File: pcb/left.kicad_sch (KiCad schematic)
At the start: 0 parts

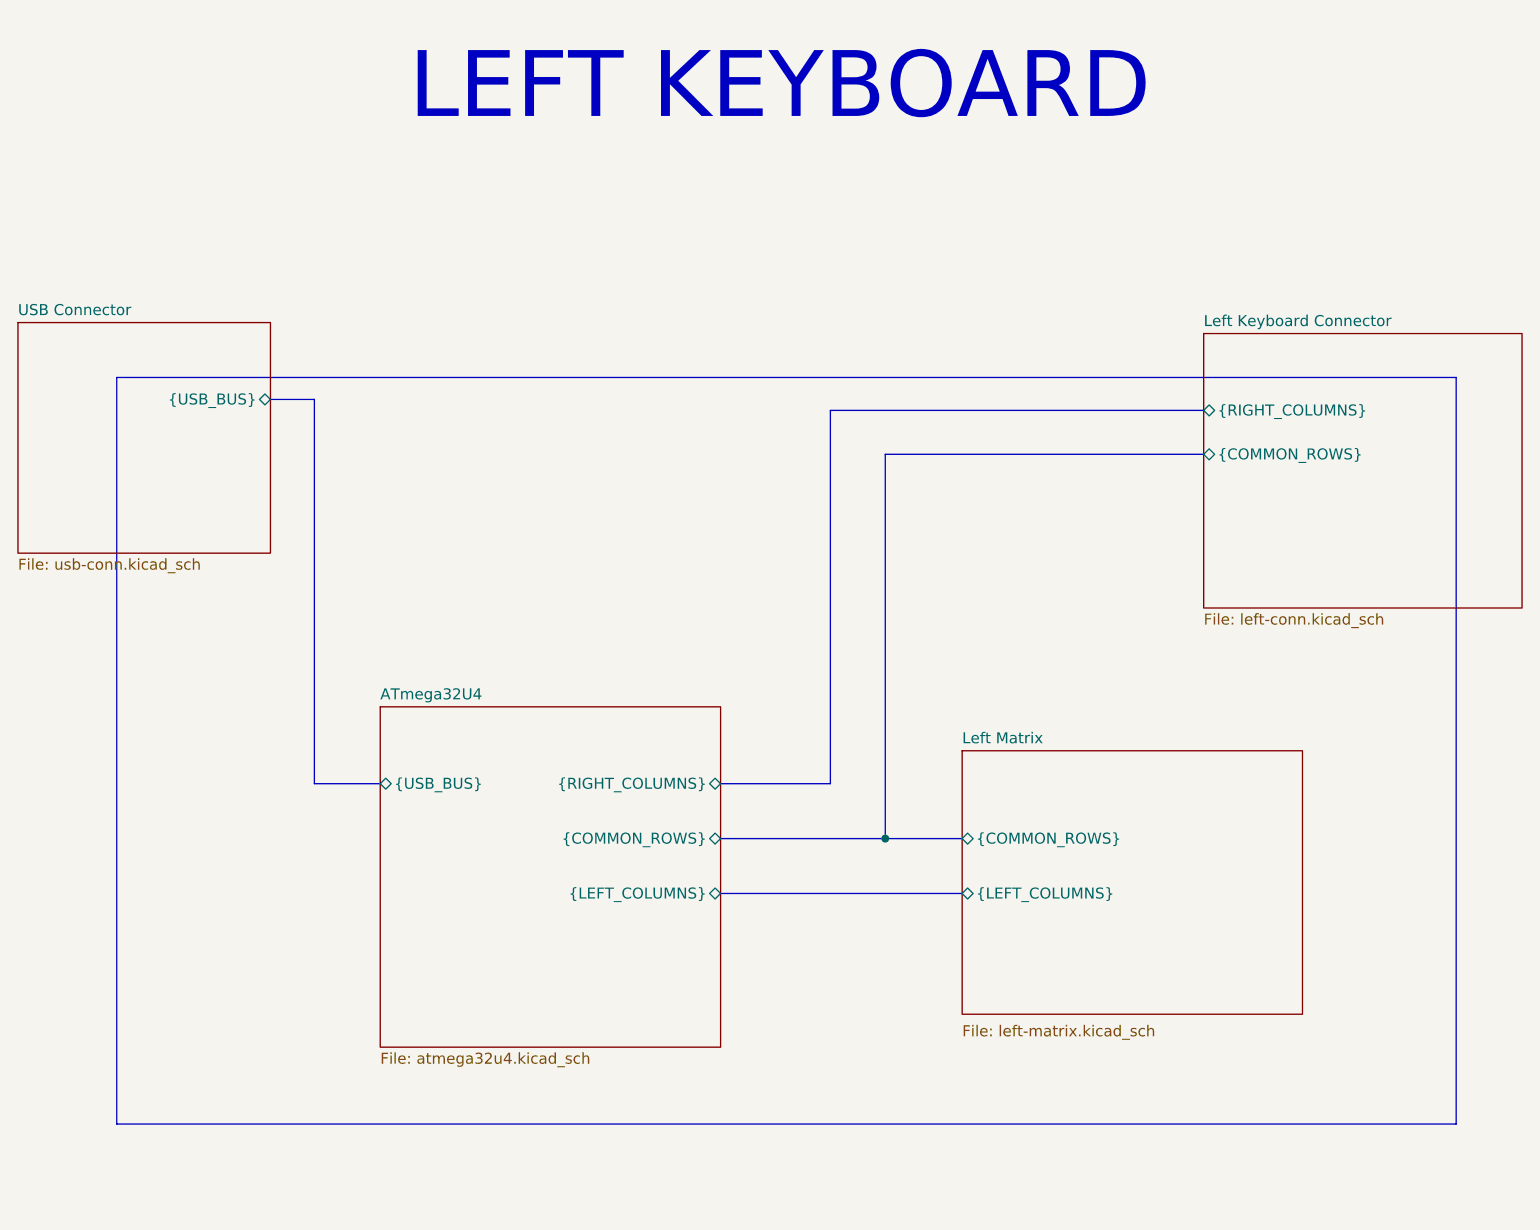
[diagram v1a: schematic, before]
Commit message: Figured out what GPIOs to use.
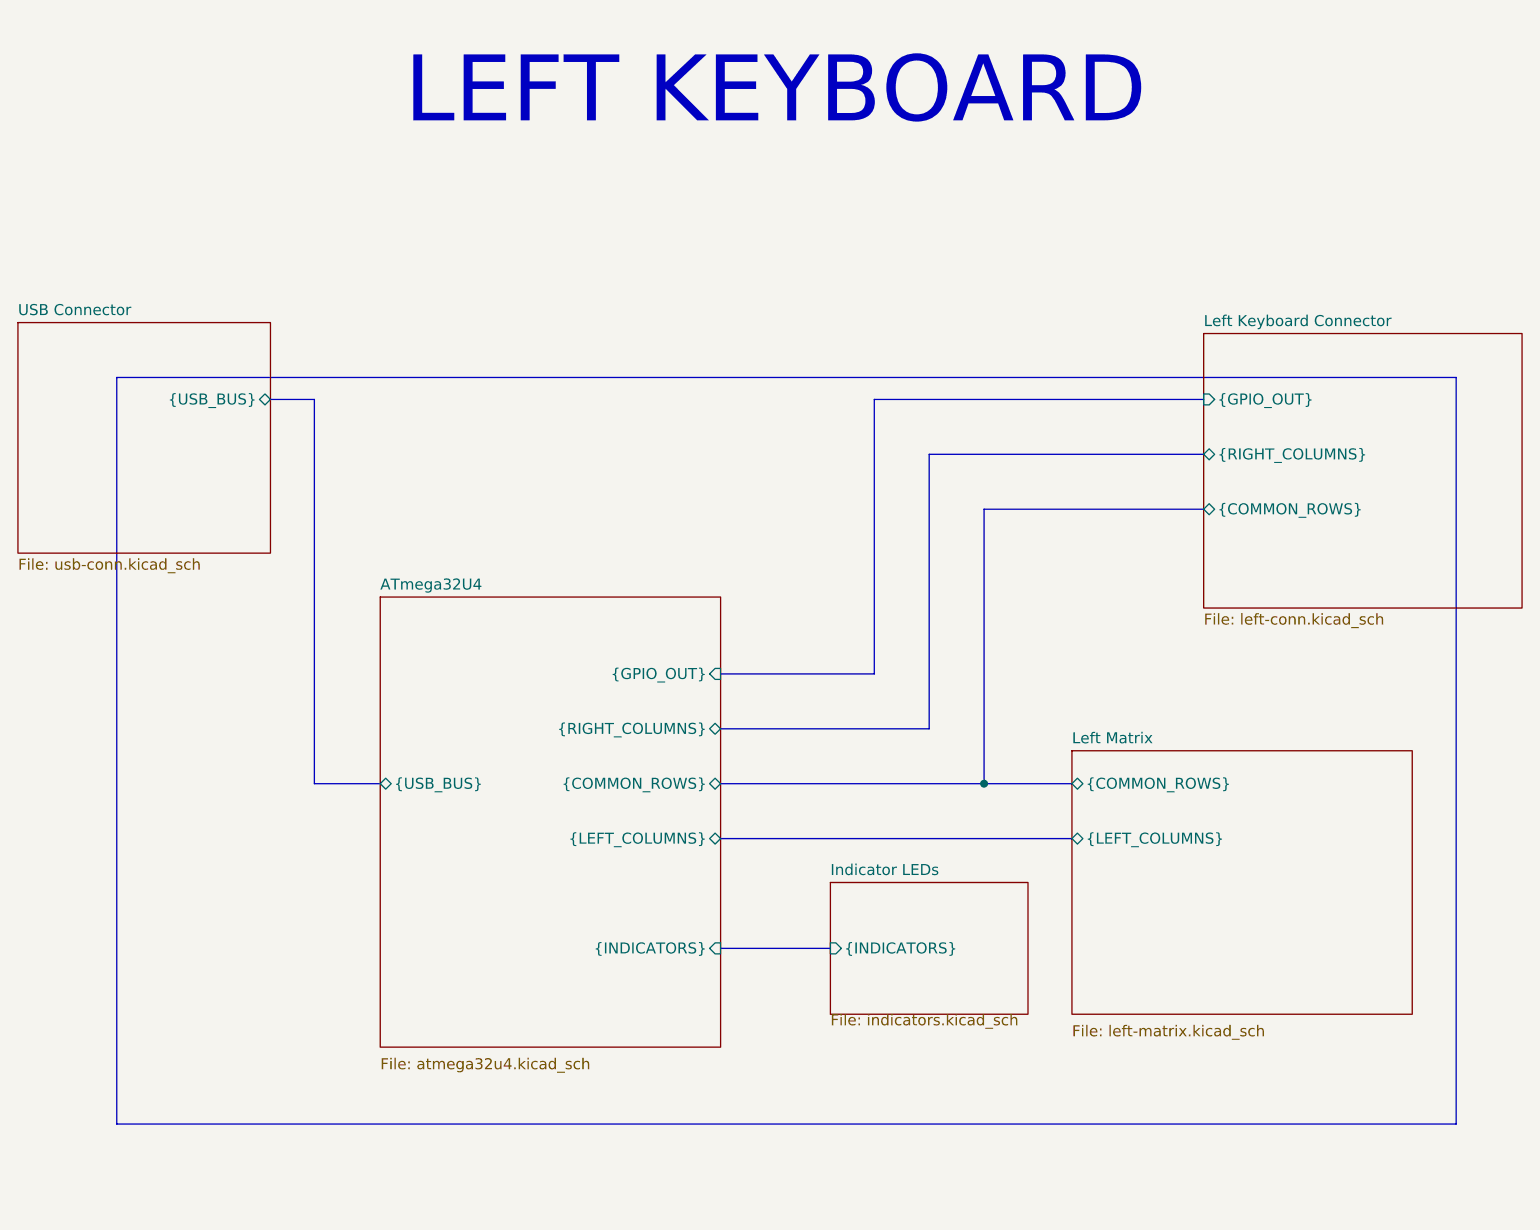
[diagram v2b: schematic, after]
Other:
- added sheet Indicator LEDs (indicators.kicad_sch)
- sheet ATmega32U4 ports: added {GPIO_OUT}, {INDICATORS}; removed none
- sheet Left Keyboard Connector ports: added {GPIO_OUT}; removed none
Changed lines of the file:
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@@
 	(text "LEFT KEYBOARD"
 		(exclude_from_sim no)
-		(at 146.558 29.972 0)
+		(at 146.05 30.48 0)
 		(effects
 			(font
@@
 	)
 	(junction
-		(at 158.75 116.84)
+		(at 170.18 110.49)
 		(diameter 0)
 		(color 0 0 0 0)
@@
 	(bus
 		(pts
-			(xy 152.4 67.31) (xy 195.58 67.31)
-		)
-		(stroke
-			(width 0)
-			(type default)
-		)
-	)
-	(bus
-		(pts
-			(xy 139.7 116.84) (xy 158.75 116.84)
+			(xy 163.83 72.39) (xy 195.58 72.39)
+		)
+		(stroke
+			(width 0)
+			(type default)
+		)
+	)
+	(bus
+		(pts
+			(xy 139.7 110.49) (xy 170.18 110.49)
 		)
 		(stroke
@@
 	(bus
 		(pts
-			(xy 139.7 123.19) (xy 167.64 123.19)
-		)
-		(stroke
-			(width 0)
-			(type default)
-		)
-	)
-	(bus
-		(pts
-			(xy 152.4 67.31) (xy 152.4 110.49)
+			(xy 139.7 116.84) (xy 180.34 116.84)
+		)
+		(stroke
+			(width 0)
+			(type default)
+		)
+	)
+	(bus
+		(pts
+			(xy 163.83 72.39) (xy 163.83 104.14)
 		)
 		(stroke
@@
 	(bus
 		(pts
-			(xy 158.75 72.39) (xy 158.75 116.84)
-		)
-		(stroke
-			(width 0)
-			(type default)
-		)
-	)
-	(bus
-		(pts
-			(xy 158.75 116.84) (xy 167.64 116.84)
-		)
-		(stroke
-			(width 0)
-			(type default)
-		)
-	)
-	(bus
-		(pts
-			(xy 139.7 110.49) (xy 152.4 110.49)
-		)
-		(stroke
-			(width 0)
-			(type default)
-		)
-	)
-	(bus
-		(pts
-			(xy 158.75 72.39) (xy 195.58 72.39)
+			(xy 157.48 97.79) (xy 157.48 66.04)
+		)
+		(stroke
+			(width 0)
+			(type default)
+		)
+	)
+	(bus
+		(pts
+			(xy 170.18 110.49) (xy 180.34 110.49)
+		)
+		(stroke
+			(width 0)
+			(type default)
+		)
+	)
+	(bus
+		(pts
+			(xy 170.18 78.74) (xy 170.18 110.49)
+		)
+		(stroke
+			(width 0)
+			(type default)
+		)
+	)
+	(bus
+		(pts
+			(xy 139.7 97.79) (xy 157.48 97.79)
+		)
+		(stroke
+			(width 0)
+			(type default)
+		)
+	)
+	(bus
+		(pts
+			(xy 139.7 129.54) (xy 152.4 129.54)
+		)
+		(stroke
+			(width 0)
+			(type default)
+		)
+	)
+	(bus
+		(pts
+			(xy 139.7 104.14) (xy 163.83 104.14)
+		)
+		(stroke
+			(width 0)
+			(type default)
+		)
+	)
+	(bus
+		(pts
+			(xy 157.48 66.04) (xy 195.58 66.04)
+		)
+		(stroke
+			(width 0)
+			(type default)
+		)
+	)
+	(bus
+		(pts
+			(xy 170.18 78.74) (xy 195.58 78.74)
 		)
 		(stroke
@@
 	)
 	(sheet
-		(at 167.64 106.68)
+		(at 180.34 106.68)
 		(size 39.37 30.48)
 		(exclude_from_sim no)
@@
 		)
 		(property "Sheetname" "Left Matrix"
-			(at 167.64 105.9684 0)
+			(at 180.34 105.9684 0)
 			(effects
 				(font
@@
 		)
 		(property "Sheetfile" "left-matrix.kicad_sch"
-			(at 167.64 138.3796 0)
+			(at 180.34 138.3796 0)
 			(effects
 				(font
@@
 		)
 		(pin "{COMMON_ROWS}" bidirectional
-			(at 167.64 116.84 180)
+			(at 180.34 110.49 180)
 			(effects
 				(font
@@
 		)
 		(pin "{LEFT_COLUMNS}" bidirectional
-			(at 167.64 123.19 180)
+			(at 180.34 116.84 180)
 			(effects
 				(font
@@
 	)
 	(sheet
-		(at 100.33 101.6)
-		(size 39.37 39.37)
+		(at 100.33 88.9)
+		(size 39.37 52.07)
 		(exclude_from_sim no)
 		(in_bom yes)
@@
 		)
 		(property "Sheetname" "ATmega32U4"
-			(at 100.33 100.8884 0)
+			(at 100.33 88.1884 0)
 			(effects
 				(font
@@
 		)
 		(property "Sheetfile" "atmega32u4.kicad_sch"
-			(at 100.33 141.5546 0)
+			(at 100.33 142.1896 0)
 			(effects
 				(font
@@
 		)
 		(pin "{COMMON_ROWS}" bidirectional
+			(at 139.7 110.49 0)
+			(effects
+				(font
+					(size 1.27 1.27)
+				)
+				(justify right)
+			)
+		)
+		(pin "{LEFT_COLUMNS}" bidirectional
 			(at 139.7 116.84 0)
 			(effects
@@
 			)
 		)
-		(pin "{LEFT_COLUMNS}" bidirectional
-			(at 139.7 123.19 0)
-			(effects
-				(font
-					(size 1.27 1.27)
-				)
-				(justify right)
-			)
-		)
 		(pin "{RIGHT_COLUMNS}" bidirectional
-			(at 139.7 110.49 0)
+			(at 139.7 104.14 0)
 			(effects
 				(font
@@
 				)
 				(justify left)
+			)
+		)
+		(pin "{GPIO_OUT}" input
+			(at 139.7 97.79 0)
+			(effects
+				(font
+					(size 1.27 1.27)
+				)
+				(justify right)
+			)
+		)
+		(pin "{INDICATORS}" input
+			(at 139.7 129.54 0)
+			(effects
+				(font
+					(size 1.27 1.27)
+				)
+				(justify right)
 			)
 		)
@@
 	)
 	(sheet
-		(at 58.42 57.15)
-		(size 29.21 26.67)
+		(at 152.4 121.92)
+		(size 22.86 15.24)
 		(exclude_from_sim no)
 		(in_bom yes)
@@
 			(color 0 0 0 0.0000)
 		)
+		(property "Sheetname" "Indicator LEDs"
+			(at 152.4 121.2084 0)
+			(effects
+				(font
+					(size 1.27 1.27)
+				)
+				(justify left bottom)
+			)
+		)
+		(property "Sheetfile" "indicators.kicad_sch"
+			(at 152.4 137.1096 0)
+			(effects
+				(font
+					(size 1.27 1.27)
+				)
+				(justify left top)
+			)
+		)
+		(pin "{INDICATORS}" input
+			(at 152.4 129.54 180)
+			(effects
+				(font
+					(size 1.27 1.27)
+				)
+				(justify left)
+			)
+		)
+		(instances
+			(project "69split"
+				(path "/d75b0717-10e3-4e20-afcb-05300684210e/a528eaf3-d99a-4f91-978f-500370d04b37"
+					(page "11")
+				)
+			)
+		)
+	)
+	(sheet
+		(at 58.42 57.15)
+		(size 29.21 26.67)
+		(exclude_from_sim no)
+		(in_bom yes)
+		(on_board yes)
+		(dnp no)
+		(fields_autoplaced yes)
+		(stroke
+			(width 0.1524)
+			(type solid)
+		)
+		(fill
+			(color 0 0 0 0.0000)
+		)
 		(property "Sheetname" "USB Connector"
 			(at 58.42 56.4384 0)
@@
 		)
 		(pin "{COMMON_ROWS}" bidirectional
+			(at 195.58 78.74 180)
+			(effects
+				(font
+					(size 1.27 1.27)
+				)
+				(justify left)
+			)
+		)
+		(pin "{RIGHT_COLUMNS}" bidirectional
 			(at 195.58 72.39 180)
 			(effects
 				(font
 					(size 1.27 1.27)
-				)
-				(justify left)
-			)
-		)
-		(pin "{RIGHT_COLUMNS}" bidirectional
-			(at 195.58 67.31 180)
-			(effects
-				(font
-					(size 1.27 1.27)
 					(thickness 0.1588)
 				)
 				(justify left)
+			)
+		)
+		(pin "{GPIO_OUT}" input
+			(at 195.58 66.04 180)
+			(effects
+				(font
+					(size 1.27 1.27)
+				)
+				(justify left)
